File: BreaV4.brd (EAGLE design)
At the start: 30.8 x 19 mm, 31 parts, among them J1 XF2L-0535-1, J2 XF2L-0535-1, Q3 ABM-16MHZ, SW1 ESE31L11T, SW2 EVQ11U09K, U1 TPS62200, X1 22-23-2021

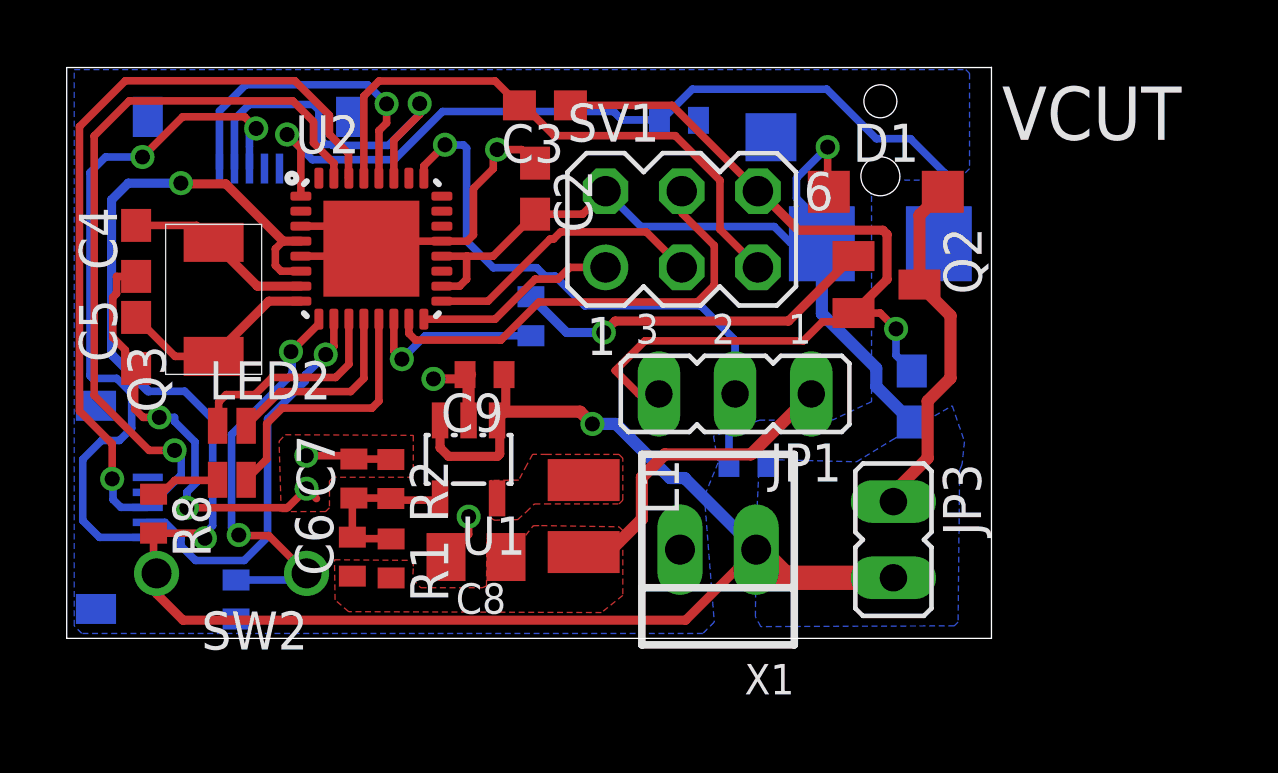
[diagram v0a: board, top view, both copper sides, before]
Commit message: Schematics/Board file commit
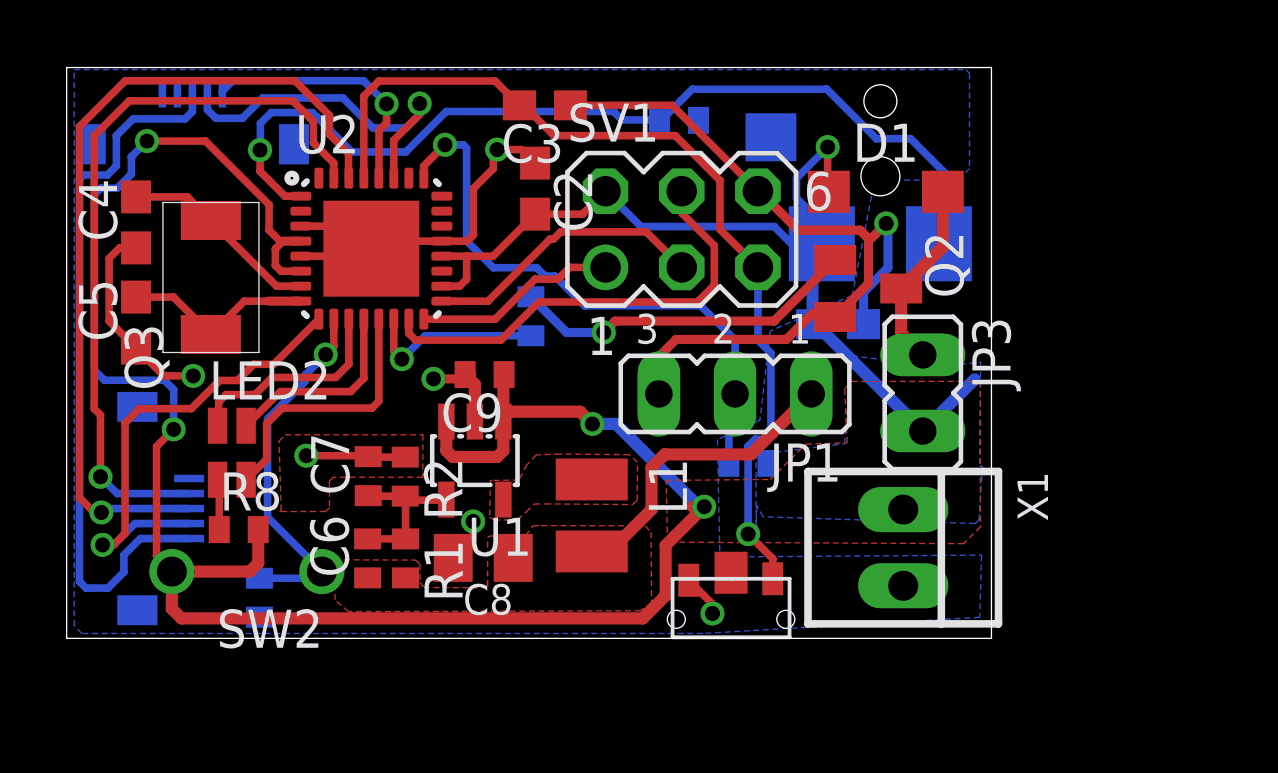
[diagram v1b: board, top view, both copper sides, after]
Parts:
- added SW3: LS12T2-T, NewPart:LS12T2-T
- moved X1 6.17 mm to (27.9, 2.99), turned to 270 degrees
- moved JP3 4.99 mm to (28.5, 8.14)
- moved C1 3.44 mm to (25.7, 10.4), turned to 0 degrees
- moved R8 2.89 mm to (5.74, 3.59), turned to 0 degrees
- moved J2 2.29 mm to (4.19, 16.3), turned to 90 degrees
- moved J1 1.38 mm to (2.18, 4.29)
- moved C4 0.95 mm to (2.32, 13.8)
- moved R7 0.78 mm to (6.43, 1.32)
- moved Q3 0.74 mm to (3.21, 9.49)
- moved C5 0.68 mm to (2.32, 10.5)
- moved Q2 0.62 mm to (26.7, 11.6)
- moved C6 0.51 mm to (10.0, 2.63)
- moved SW2 0.51 mm to (6.01, 2.19)
- moved C7 0.49 mm to (10.1, 5.37)
- moved R2 0.49 mm to (11.3, 5.36)
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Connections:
- net GND: now also SW3.P$1
- net PWRSW: now also U2.10; no longer U2.9
- net REST: now also U2.9; no longer U2.10
- net RST: now also SW3.P$2
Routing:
- net RST: track 19.7 -> 31.1 mm, vias 0 -> 1
- net GND: track 66.1 -> 57.2 mm, vias 8 -> 7
- net N$9: track 11.9 -> 6.31 mm
- net REST: track 13.2 -> 15.7 mm
- net DETSW: track 29.3 -> 31.5 mm
- net RX: track 26.0 -> 28.1 mm
- net SCL: track 10.7 -> 8.56 mm
- net VCC: track 97.6 -> 99.2 mm, vias 4 -> 5
- net PWRSW: track 13.8 -> 12.3 mm, vias 2 -> 1
- net SDA: track 12.8 -> 11.9 mm
- net N$10: track 12.3 -> 11.6 mm
- net N$5: track 2.33 -> 1.68 mm
- net VBATSIM: track 24.0 -> 24.1 mm, vias 2 -> 0
- added copper zone on layer 1, net VCC
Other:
- board text removed: "VCUT"
